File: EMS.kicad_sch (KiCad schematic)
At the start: 19 parts, among them J9 Conn_01x02_Socket, Q10 2SC2712-GR_TE85L,F, Q8 2SA1162-GR_F_, Q9 2SC2712-GR_TE85L,F, SW1 SW_MEC_5G, SW2 SW_MEC_5G

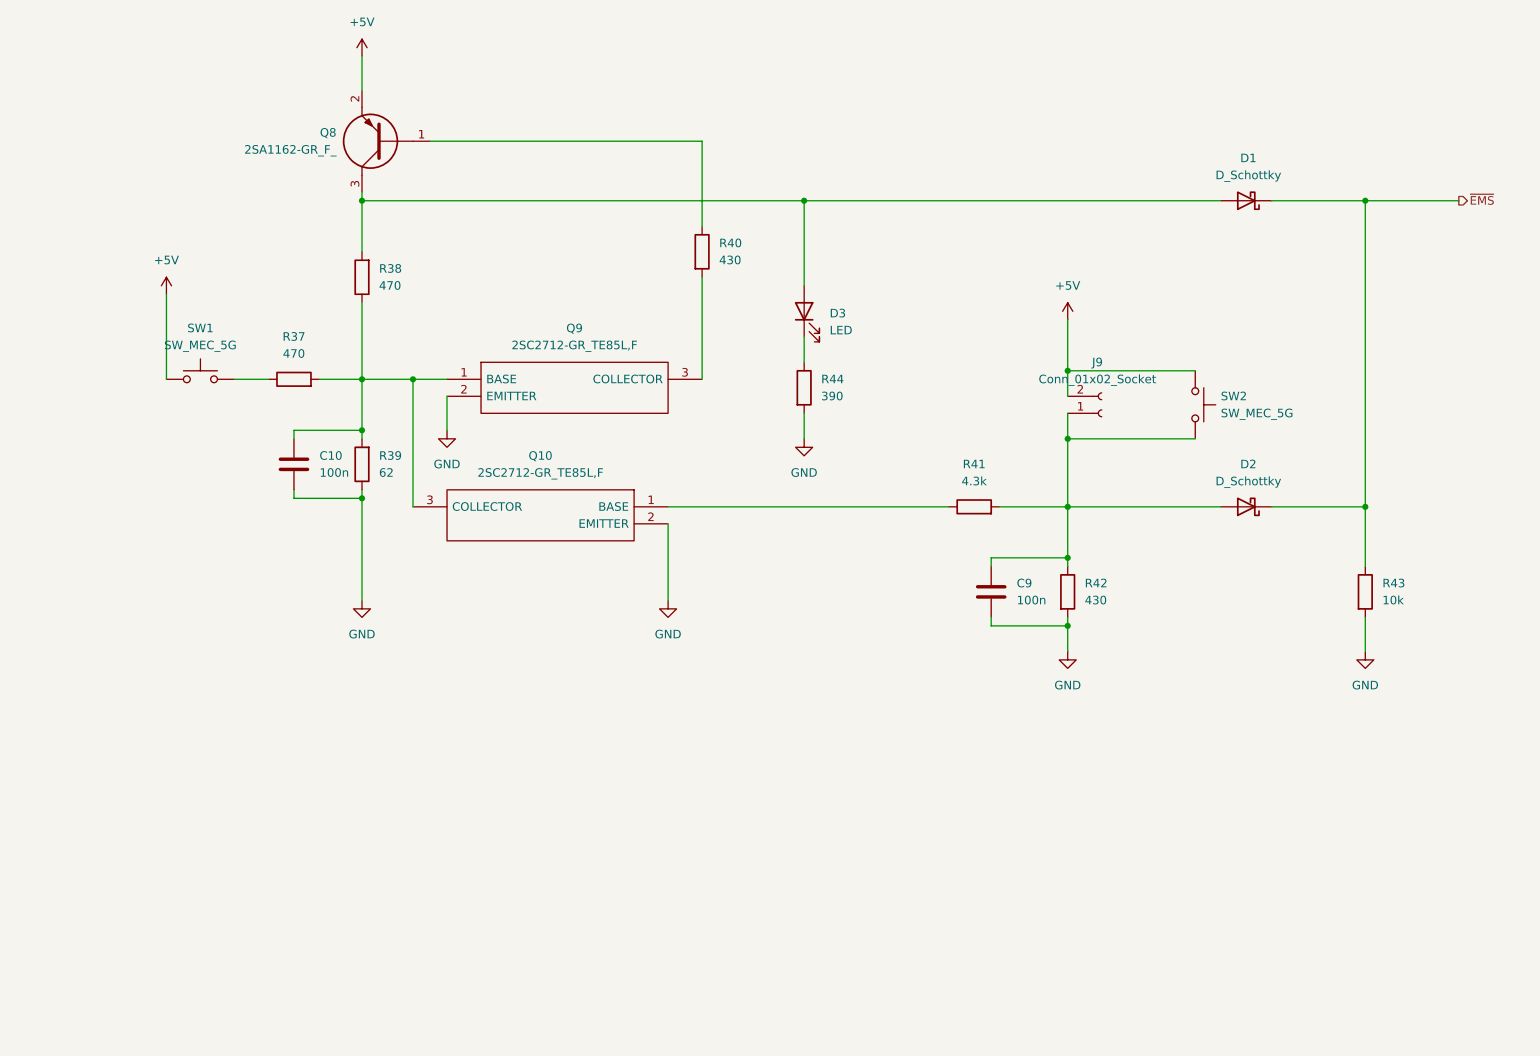
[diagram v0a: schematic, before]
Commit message: CircuitComplete
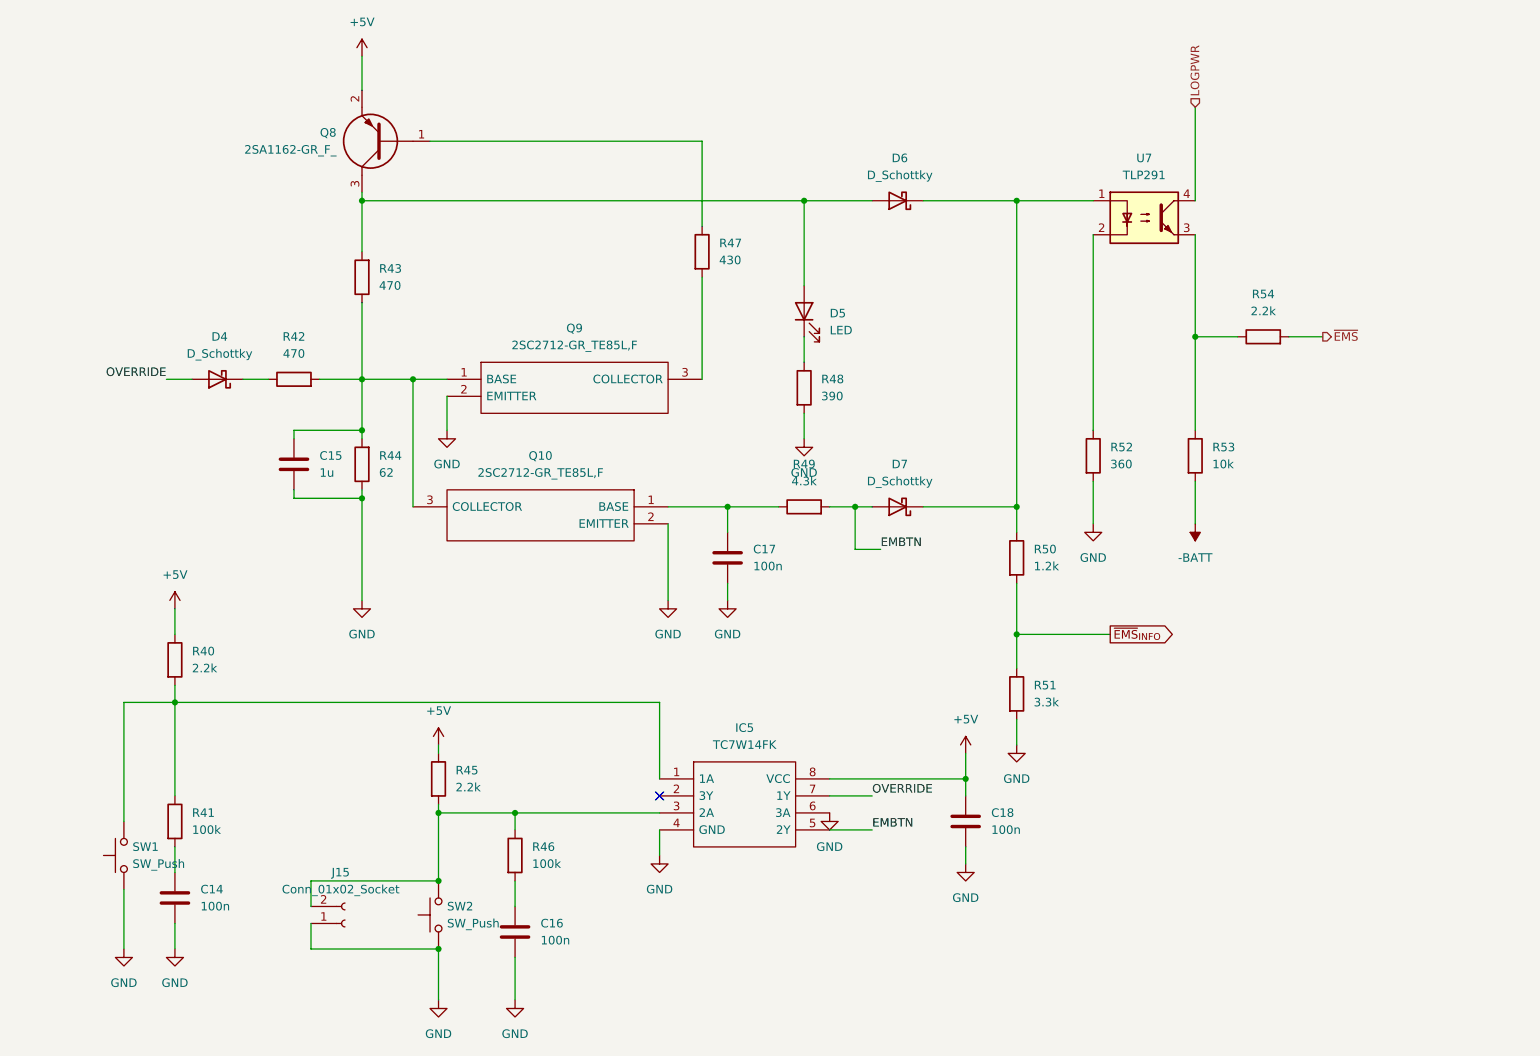
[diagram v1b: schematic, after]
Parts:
- removed C9: 100n, Capacitor_SMD:C_0603_1608Metric, symbol Device:C
- removed R43: 10k, Resistor_SMD:R_0603_1608Metric, symbol Device:R
- removed SW1, SW2: SW_MEC_5G, Button_Switch_THT:SW_PUSH_6mm, symbol Switch:SW_MEC_5G
- added C14, C16, C17, C18: 100n, Capacitor_SMD:C_0603_1608Metric, symbol Device:C
- added D4: D_Schottky, Diode_SMD:D_SOD-323, symbol Device:D_Schottky
- added IC5: TC7W14FK, SamacSys_Parts:SOP50P310X90-8N, symbol SamacSys_Parts:TC7W14FK
- added R40, R54: 2.2k, Resistor_SMD:R_0603_1608Metric, symbol Device:R
- added R41, R46: 100k, Resistor_SMD:R_0603_1608Metric, symbol Device:R
- added R50: 1.2k, Resistor_SMD:R_0603_1608Metric, symbol Device:R
- added R51: 3.3k, Resistor_SMD:R_0603_1608Metric, symbol Device:R
- added R52: 360, Resistor_SMD:R_0603_1608Metric, symbol Device:R
- added R53: 10k, Resistor_SMD:R_0603_1608Metric, symbol Device:R
- added SW1, SW2: SW_Push, Button_Switch_THT:SW_PUSH_6mm_H4.3mm, symbol Switch:SW_Push
- added U7: TLP291, Package_SO:SOIC-4_4.55x2.6mm_P1.27mm, symbol Isolator:TLP291
- C15: renamed from C10; value 100n -> 1u
- R45: renamed from R42; value 430 -> 2.2k
- renumbered D3 to D5, D1 to D6, D2 to D7, J9 to J15, R37 to R42, R38 to R43, R39 to R44, R40 to R47, R44 to R48, R41 to R49
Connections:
- net +5V: now also R45.1, C18.1, IC5.8 (VCC), R40.1; no longer J15.2 (Pin_2)
- net GND: now also J15.1 (Pin_1), C14.2, C16.2, C17.2, C18.2, IC5.4 (GND), IC5.6 (3A), R51.2, R52.2, SW1.1, SW2.1; no longer R45.2
- net ~{EMS}: now also R54.2; no longer D6.1 (K), D7.1 (K)
- net at R42.1: now also D4.1 (K)
- net EMBTN: now reaches D7.2 (A), R49.2
- net EMBTN: now also IC5.5 (2Y); no longer J15.1 (Pin_1), R45.1
- net at Q10.1 (BASE), R49.1: now also C17.1
- new net: D6.1 (K), D7.1 (K), R50.1, U7.1
- new net: C16.1, R46.2
- new net: IC5.3 (2A), J15.2 (Pin_2), R45.2, R46.1, SW2.2
- new net: C14.1, R41.2
- new net: R53.1, R54.1, U7.3
- new net: IC5.1 (1A), R40.2, R41.1, SW1.2
- new net: R52.1, U7.2
- new net -BATT: R53.2
- new net LOGPWR: U7.4
- new net OVERRIDE: D4.2 (A), IC5.7 (1Y)
- new net ~{EMS}_{INFO}: R50.2, R51.1
- no-connect marks 0 -> 1
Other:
- moved on the sheet: D6, D7, J15, R45, R49

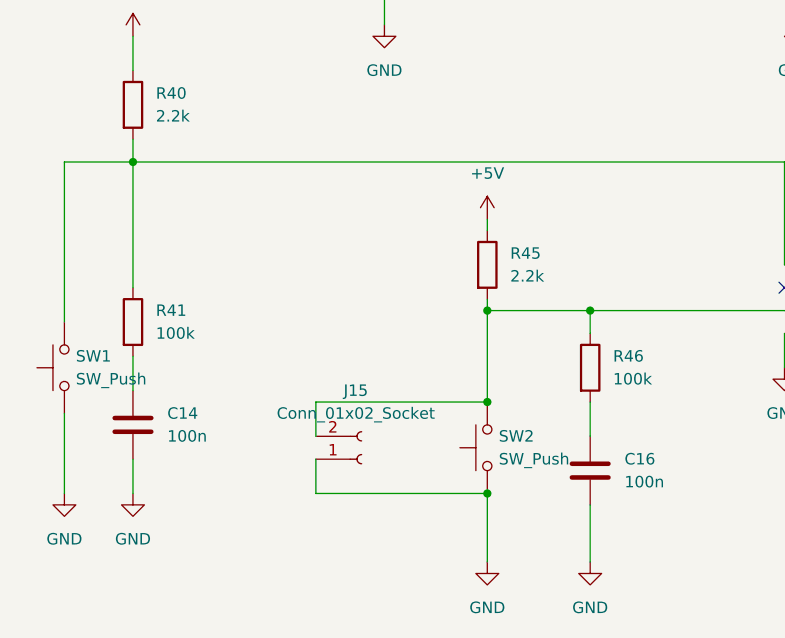
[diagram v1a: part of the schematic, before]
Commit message: Rev1
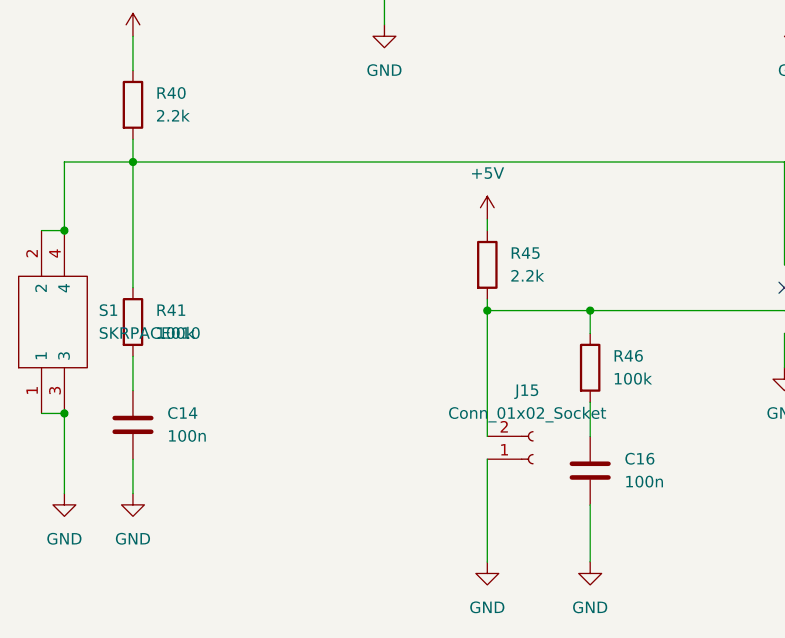
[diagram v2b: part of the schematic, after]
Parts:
- removed SW1, SW2: SW_Push, Button_Switch_THT:SW_PUSH_6mm_H4.3mm, symbol Switch:SW_Push
- added S1: SKRPACE010, SamacSys_Parts:SMT_4.2X3.2_, symbol SamacSys_Parts:SKRPACE010
- J15: footprint Connector_JST:JST_XH_B2B-XH-AM_1x02_P2.50mm_Vertical -> Connector_JST:JST_XH_B2B-XH-A_1x02_P2.50mm_Vertical
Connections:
- net GND: now also S1.1, S1.3
- net at IC5.1 (1A), R40.2, R41.1: now also S1.2, S1.4
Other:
- moved on the sheet: J15

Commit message: Rev1
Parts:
- D4: footprint Diode_SMD:D_SOD-323 -> Diode_SMD:D_SOD-323F; JLCPCB Parts# (none) -> C50704
- D6, D7: JLCPCB Parts# (none) -> C50704
- Q10, Q9: JLCPCB Parts# (none) -> C83447
- Q8: footprint SamacSys_Parts:SSM3K7002CFULF -> Package_TO_SOT_SMD:SC-59; JLCPCB Parts# (none) -> C155455
- U7: JLCPCB Parts# (none) -> C5121290

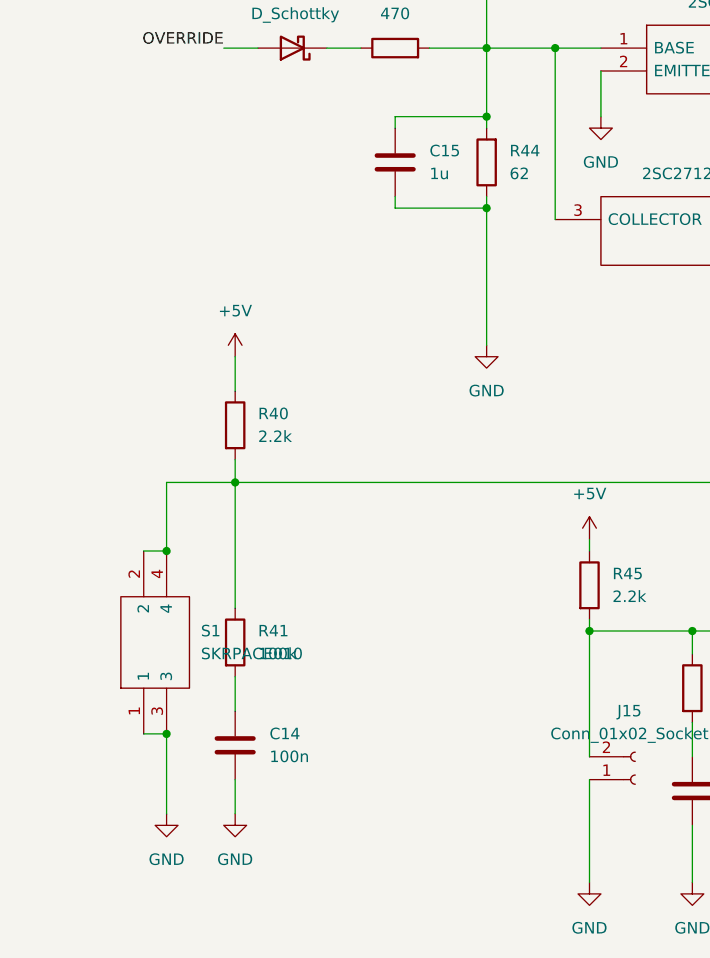
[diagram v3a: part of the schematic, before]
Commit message: Rev1.1
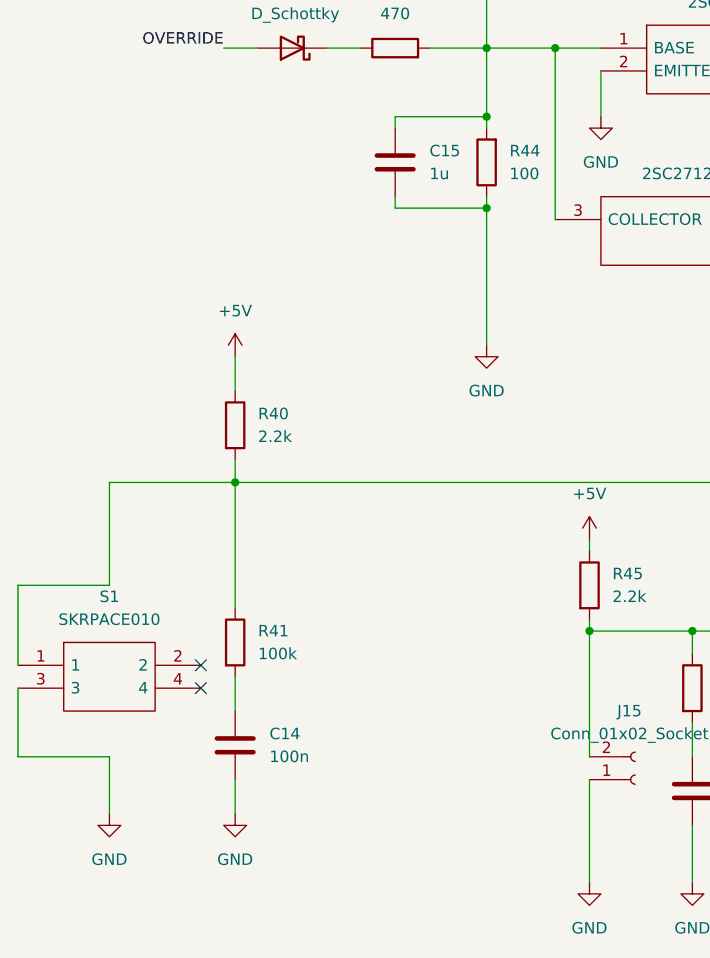
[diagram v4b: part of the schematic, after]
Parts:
- R44: value 62 -> 100
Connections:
- net GND: no longer S1.1
- net at IC5.1 (1A), R40.2, R41.1: now also S1.1; no longer S1.2, S1.4
- no-connect marks 1 -> 3
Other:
- moved on the sheet: S1
